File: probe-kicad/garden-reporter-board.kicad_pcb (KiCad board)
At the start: 2 copper layers, 40.6 x 88.9 mm, 22 parts, among them J1 70543-0106, J2 Conn_01x02, J3 70543-0002, J4 70543-0002, J5 70543-0002, Q1 TN0702N3-G, U1 MCP1700-3302E_TO92, U2 MCP1700-3302E_TO92

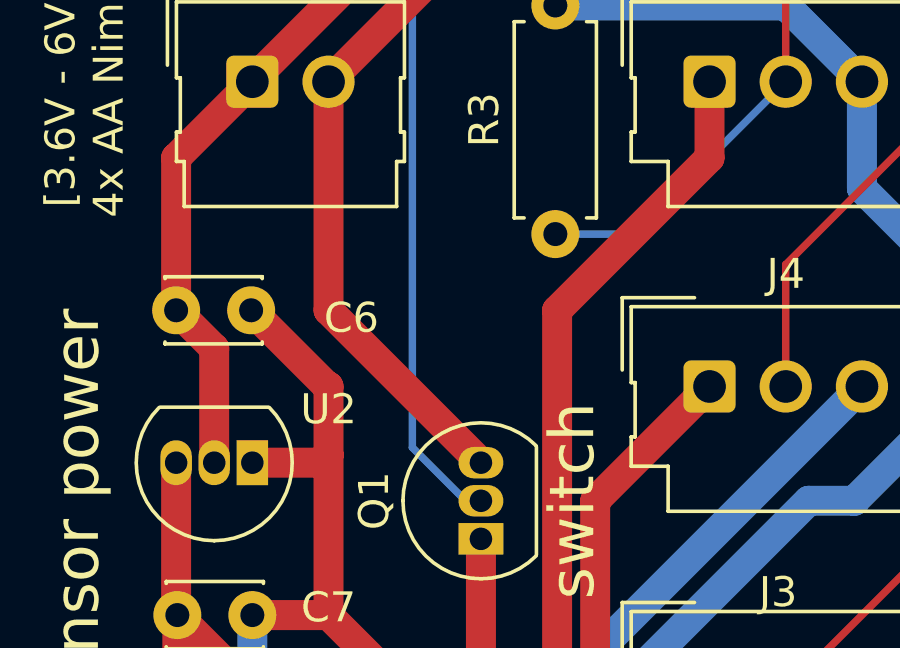
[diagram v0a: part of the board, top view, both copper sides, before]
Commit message: Feature/better doc
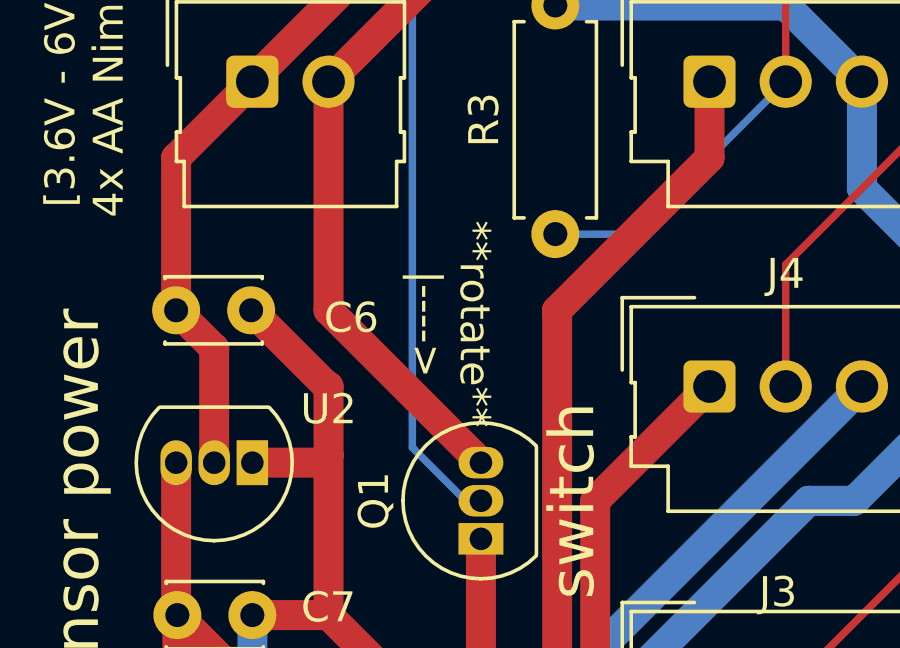
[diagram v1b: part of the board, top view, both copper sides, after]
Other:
- board text added: "**rotate** |---->"
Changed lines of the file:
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@@
     (effects (font (size 1.5 1.5) (thickness 0.3)))
+  )
+  (gr_text "**rotate**\n|---->" (at 150.114 121.1072 270) (layer "F.SilkS")
+    (effects (font (size 1 1) (thickness 0.15)))
   )
   (gr_text "Light" (at 170.18 112.776 90) (layer "F.SilkS")
